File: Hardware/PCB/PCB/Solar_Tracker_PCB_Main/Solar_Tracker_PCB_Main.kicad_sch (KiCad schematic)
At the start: 0 parts

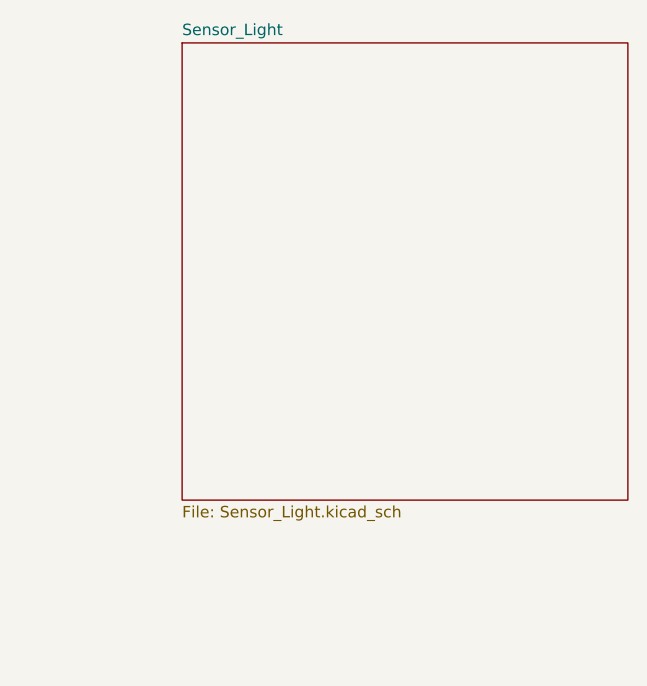
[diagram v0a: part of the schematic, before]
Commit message: actualizacion de pcb (IMU)
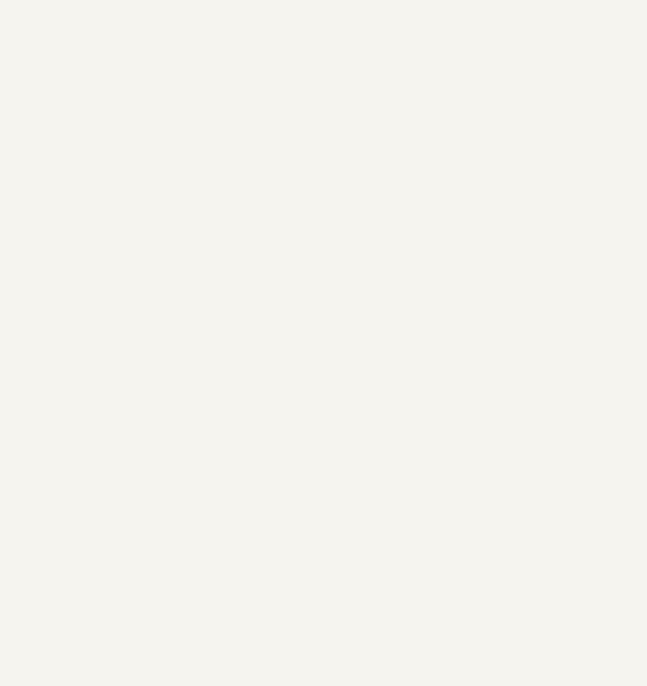
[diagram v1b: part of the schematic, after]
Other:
- removed sheet Sensor_Light
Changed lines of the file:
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@@
-		)
-	)
-	(sheet
-		(at 152.4 27.94)
-		(size 49.53 50.8)
-		(exclude_from_sim no)
-		(in_bom yes)
-		(on_board yes)
-		(dnp no)
-		(fields_autoplaced yes)
-		(stroke
-			(width 0.1524)
-			(type solid)
-		)
-		(fill
-			(color 0 0 0 0.0000)
-		)
-		(property "Sheetname" "Sensor_Light"
-			(at 152.4 27.2284 0)
-			(effects
-				(font
-					(size 1.27 1.27)
-				)
-				(justify left bottom)
-			)
-		)
-		(property "Sheetfile" "Sensor_Light.kicad_sch"
-			(at 152.4 79.3246 0)
-			(effects
-				(font
-					(size 1.27 1.27)
-				)
-				(justify left top)
-			)
-		)
-		(instances
-			(project "Solar_Tracker_PCB_Main"
-				(path "/99b6ddd9-7ffe-4c85-972a-e0f594a166d4"
-					(page "3")
-				)
-			)
 		)
 	)
